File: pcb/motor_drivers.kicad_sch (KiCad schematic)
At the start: 12 parts, among them U5 DRV8837, U6 DRV8837, U7 DRV8837, U8 DRV8837

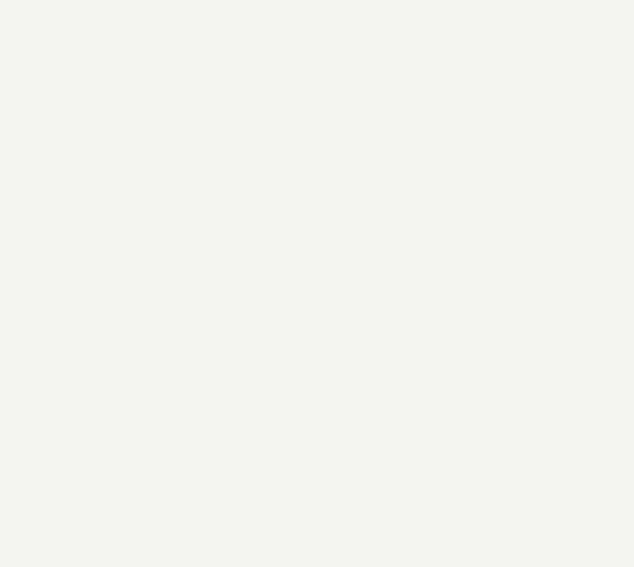
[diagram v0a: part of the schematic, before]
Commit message: WIP on the motor driver board
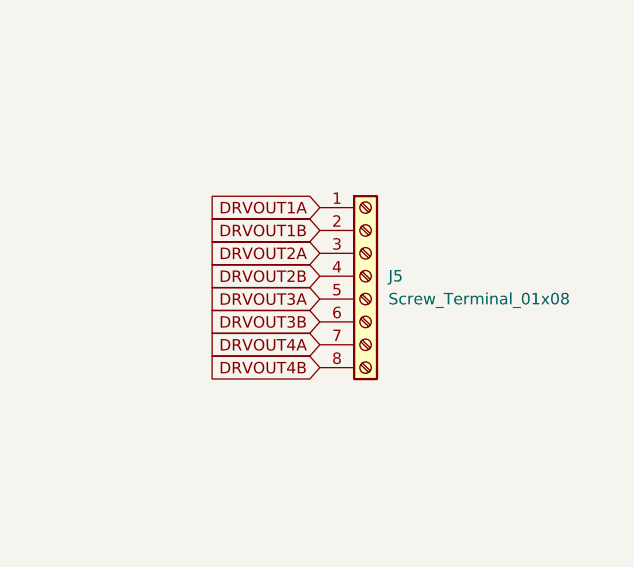
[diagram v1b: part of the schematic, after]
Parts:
- added J5: Screw_Terminal_01x08, TerminalBlock_Phoenix:TerminalBlock_Phoenix_MKDS-1,5-8-5.08_1x08_P5.08mm_Horizontal, symbol Connector:Screw_Terminal_01x08
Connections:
- net DRVOUT1A: now also J5.1 (Pin_1)
- net DRVOUT1B: now also J5.2 (Pin_2)
- net DRVOUT2A: now also J5.3 (Pin_3)
- net DRVOUT2B: now also J5.4 (Pin_4)
- net DRVOUT3A: now also J5.5 (Pin_5)
- net DRVOUT3B: now also J5.6 (Pin_6)
- net DRVOUT4A: now also J5.7 (Pin_7)
- net DRVOUT4B: now also J5.8 (Pin_8)
